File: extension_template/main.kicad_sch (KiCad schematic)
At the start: 17 parts, among them J6 MISC

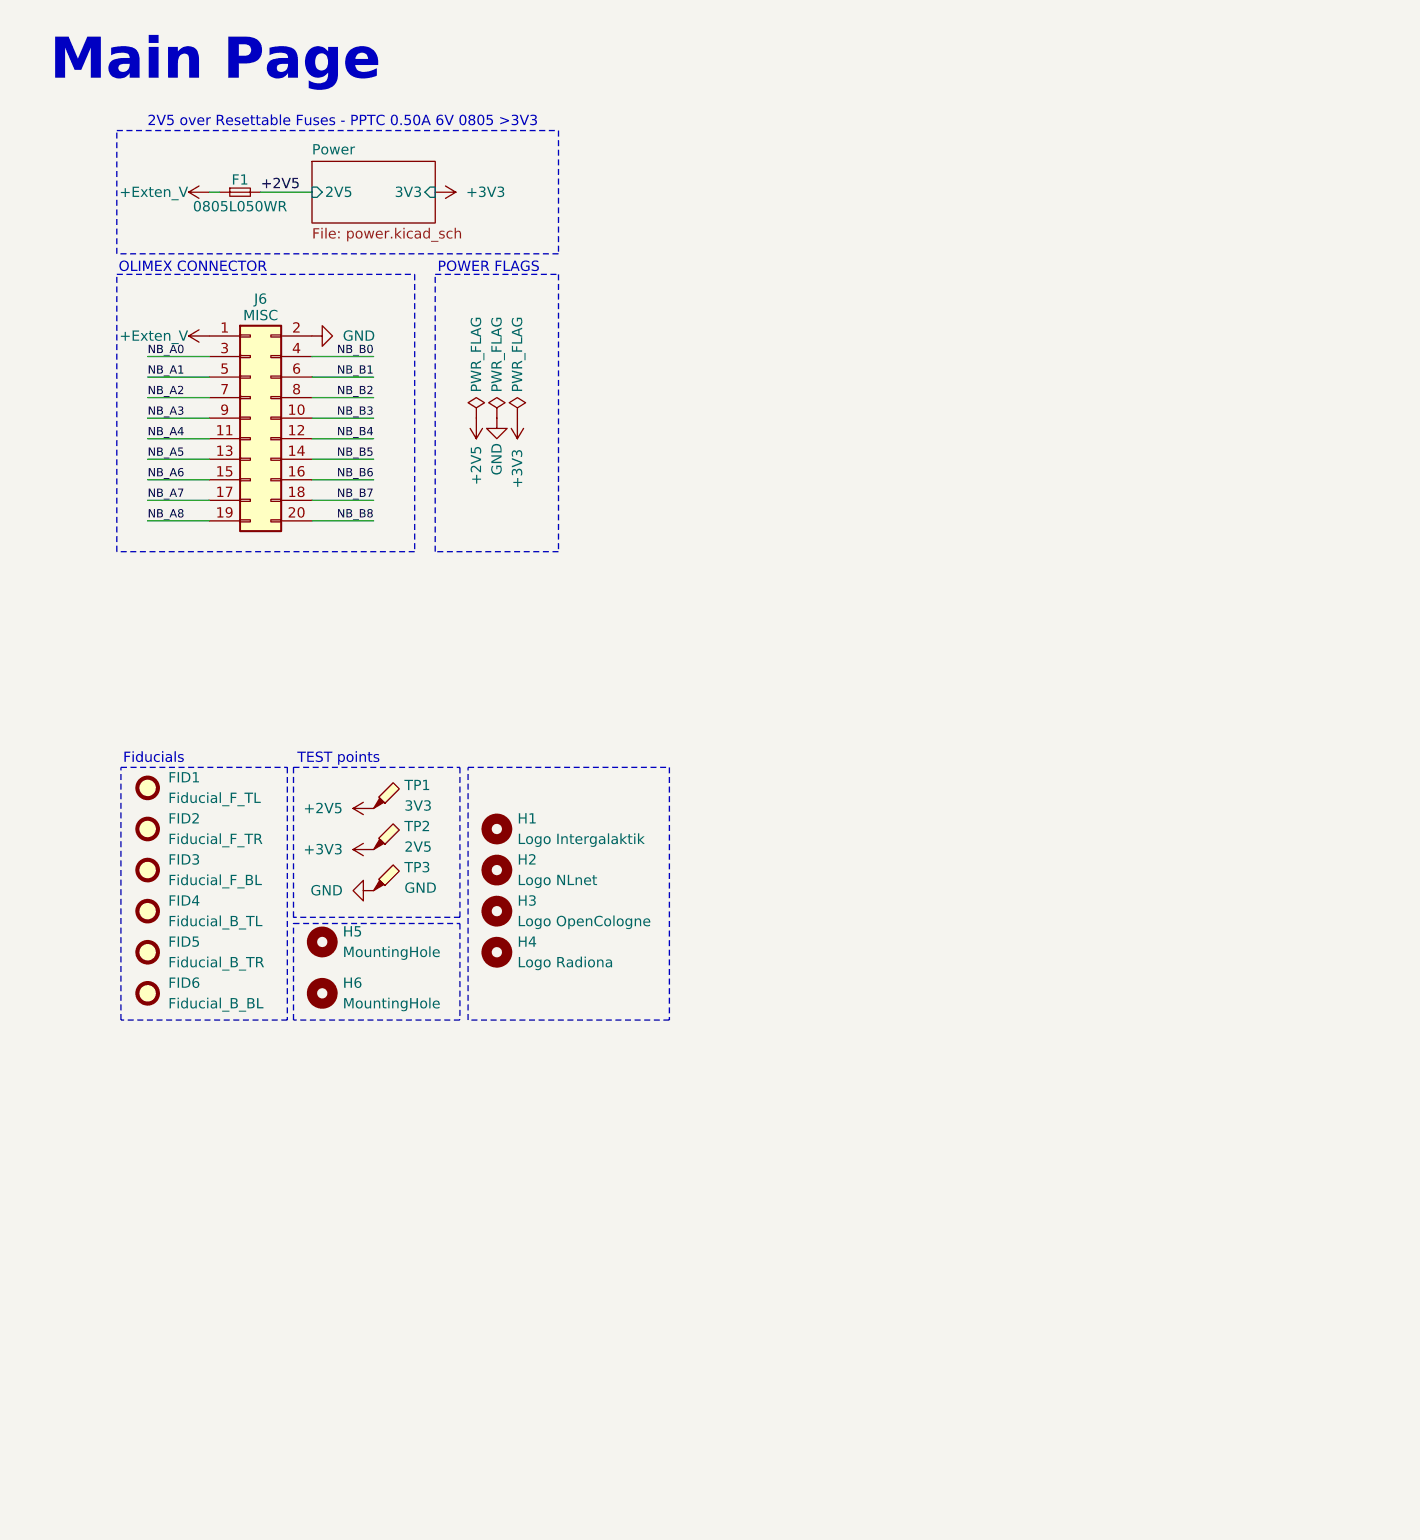
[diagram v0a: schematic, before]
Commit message: Template update
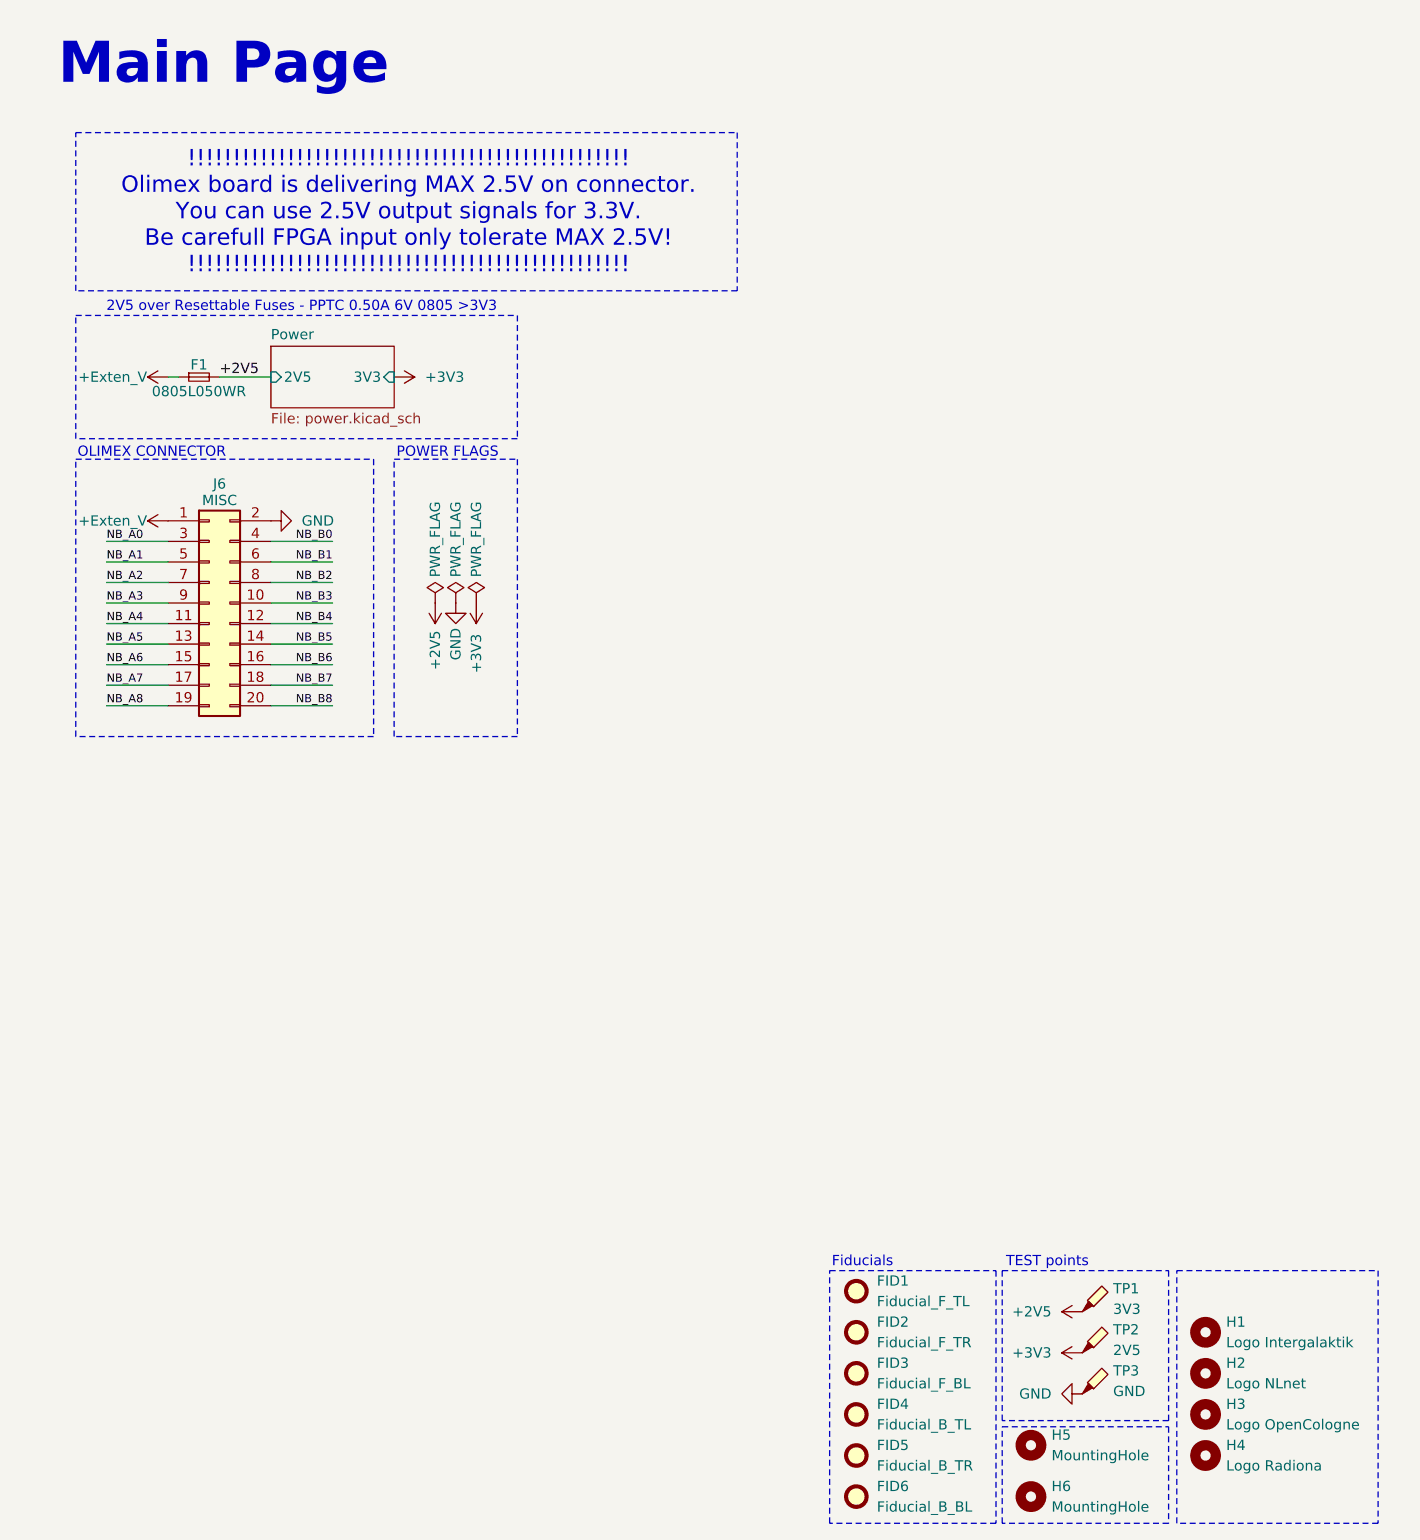
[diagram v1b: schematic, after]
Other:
- note added: "!!!!!!!!!!!!!!!!!!!!!!!!!!!!!!!!!!!!!!!!!!!!!!!!! Olimex board is delivering MAX 2.5V on connector. You can use 2.5V output signals for 3.3V. Be carefull FPGA input only tolerate MAX 2.5V! !!!!!!!!!!!!!!!!!!!!!!!!!!!!!!!!!!!!!!!!!!!!!!!!!"
- moved on the sheet: F1, FID1, FID2, FID3, FID4, FID5, FID6, H1, H2, H3, H4, H5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

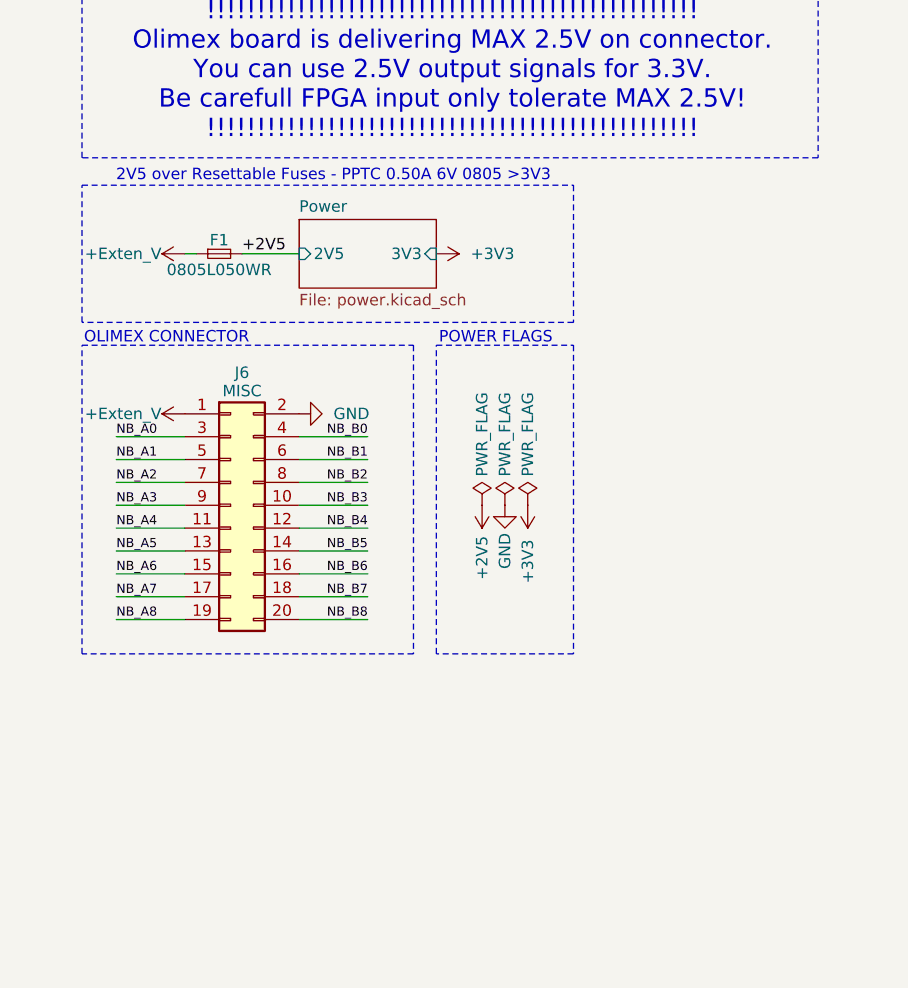
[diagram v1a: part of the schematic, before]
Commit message: Template update
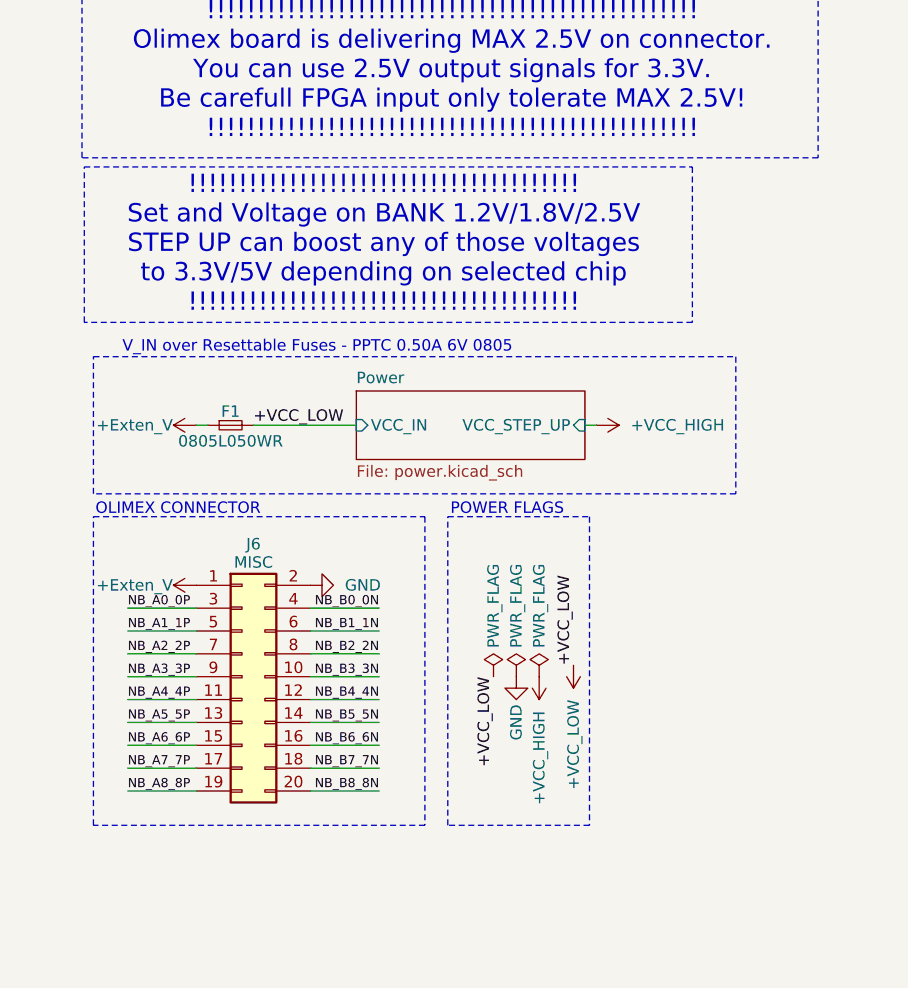
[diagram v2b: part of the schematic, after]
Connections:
- net +2V5: no longer F1.2
- net NB_A0 renamed NB_A0_0P
- net NB_A1 renamed NB_A1_1P
- net NB_A2 renamed NB_A2_2P
- net NB_A3 renamed NB_A3_3P
- net NB_A4 renamed NB_A4_4P
- net NB_A5 renamed NB_A5_5P
- net NB_A6 renamed NB_A6_6P
- net NB_A7 renamed NB_A7_7P
- net NB_A8 renamed NB_A8_8P
- net NB_B0 renamed NB_B0_0N
- net NB_B1 renamed NB_B1_1N
- net NB_B2 renamed NB_B2_2N
- net NB_B3 renamed NB_B3_3N
- net NB_B4 renamed NB_B4_4N
- net NB_B5 renamed NB_B5_5N
- net NB_B6 renamed NB_B6_6N
- net NB_B7 renamed NB_B7_7N
- net NB_B8 renamed NB_B8_8N
- new net +VCC_LOW: F1.2
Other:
- sheet Power ports: added VCC_IN, VCC_STEP_UP; removed 2V5, 3V3
- note added: "!!!!!!!!!!!!!!!!!!!!!!!!!!!!!!!!!!!!!!! Set and Voltage on BANK 1.2V/1.8V/2.5V STEP UP can boost any of those voltages to 3.3V/5V depending on selected chip !!!!!!!!!!!!!!!!!!!!!!!!!!!!!!!!!!!!!!!"
- note added: "V_IN over Resettable Fuses - PPTC 0.50A 6V 0805"
- note removed: "2V5 over Resettable Fuses - PPTC 0.50A 6V 0805 >3V3"
- moved on the sheet: F1, J6
